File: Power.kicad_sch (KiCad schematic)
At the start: 26 parts, among them J401 KLDX-0202-B, J402 EBWA-02-B, Q401 MCU18P10Y-TP, U401 TPS7A2030PDBVR

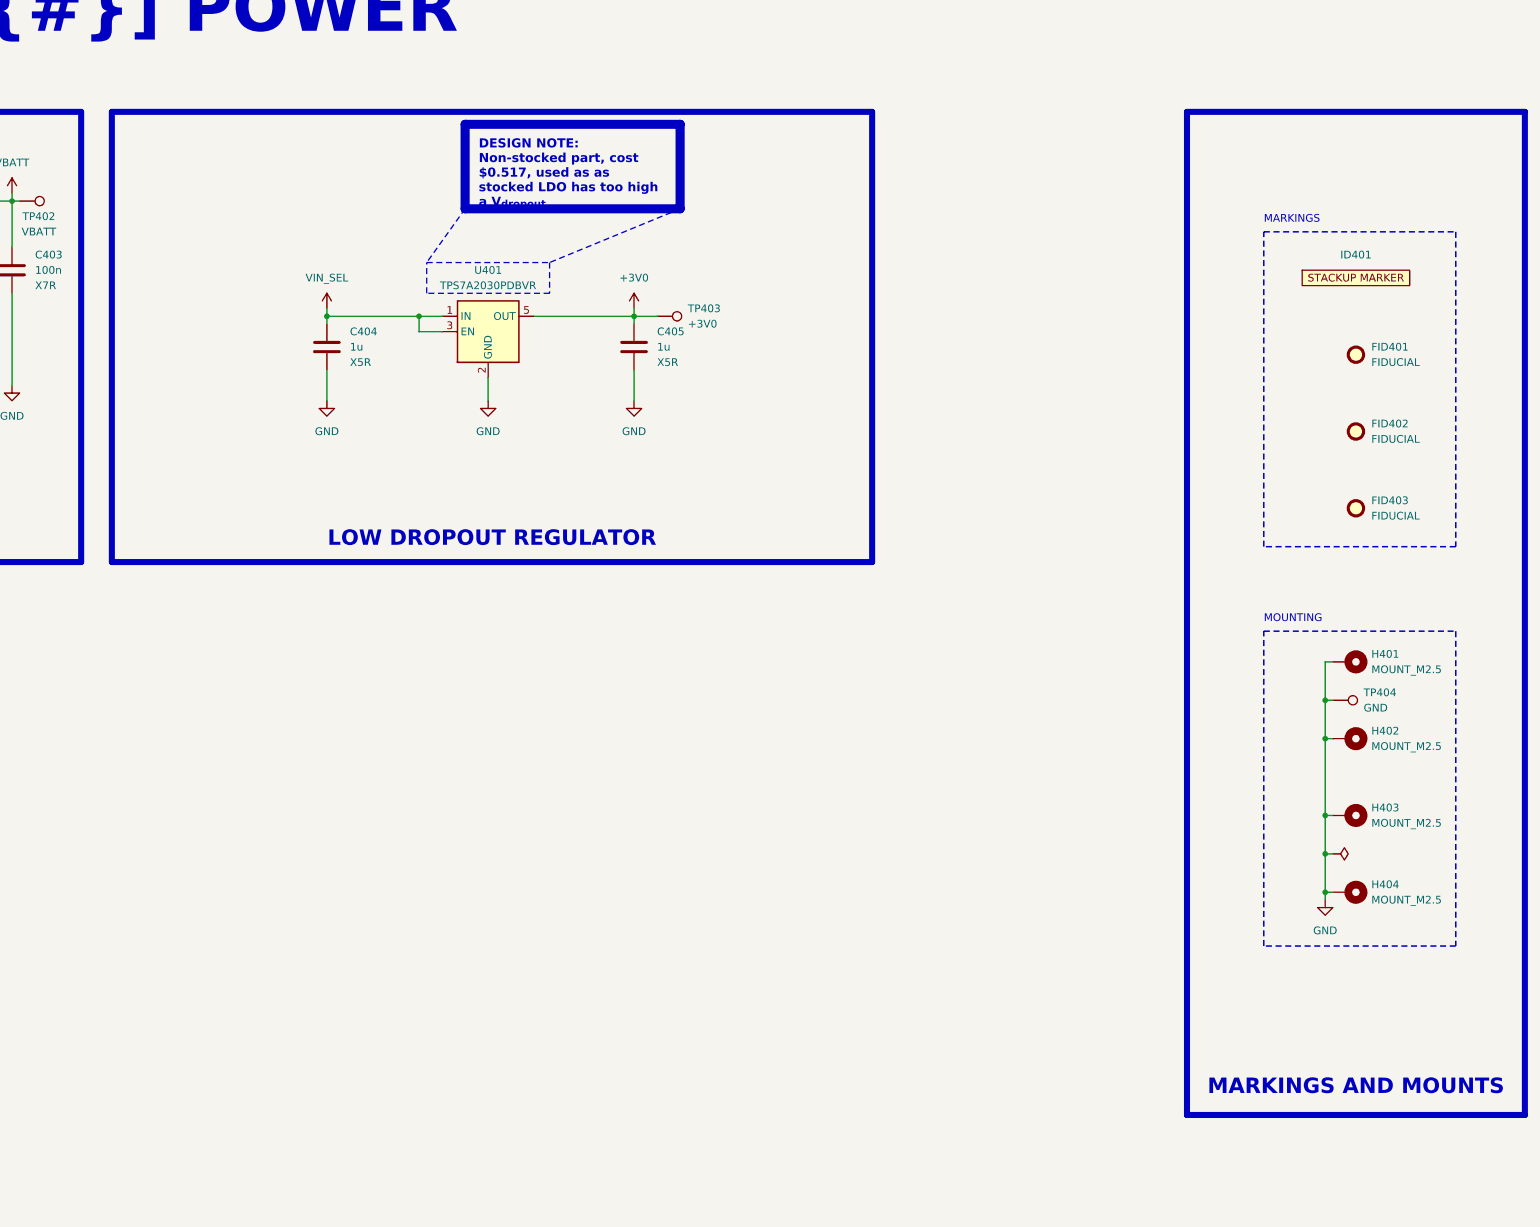
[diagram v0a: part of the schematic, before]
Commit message: feat: checked REV A
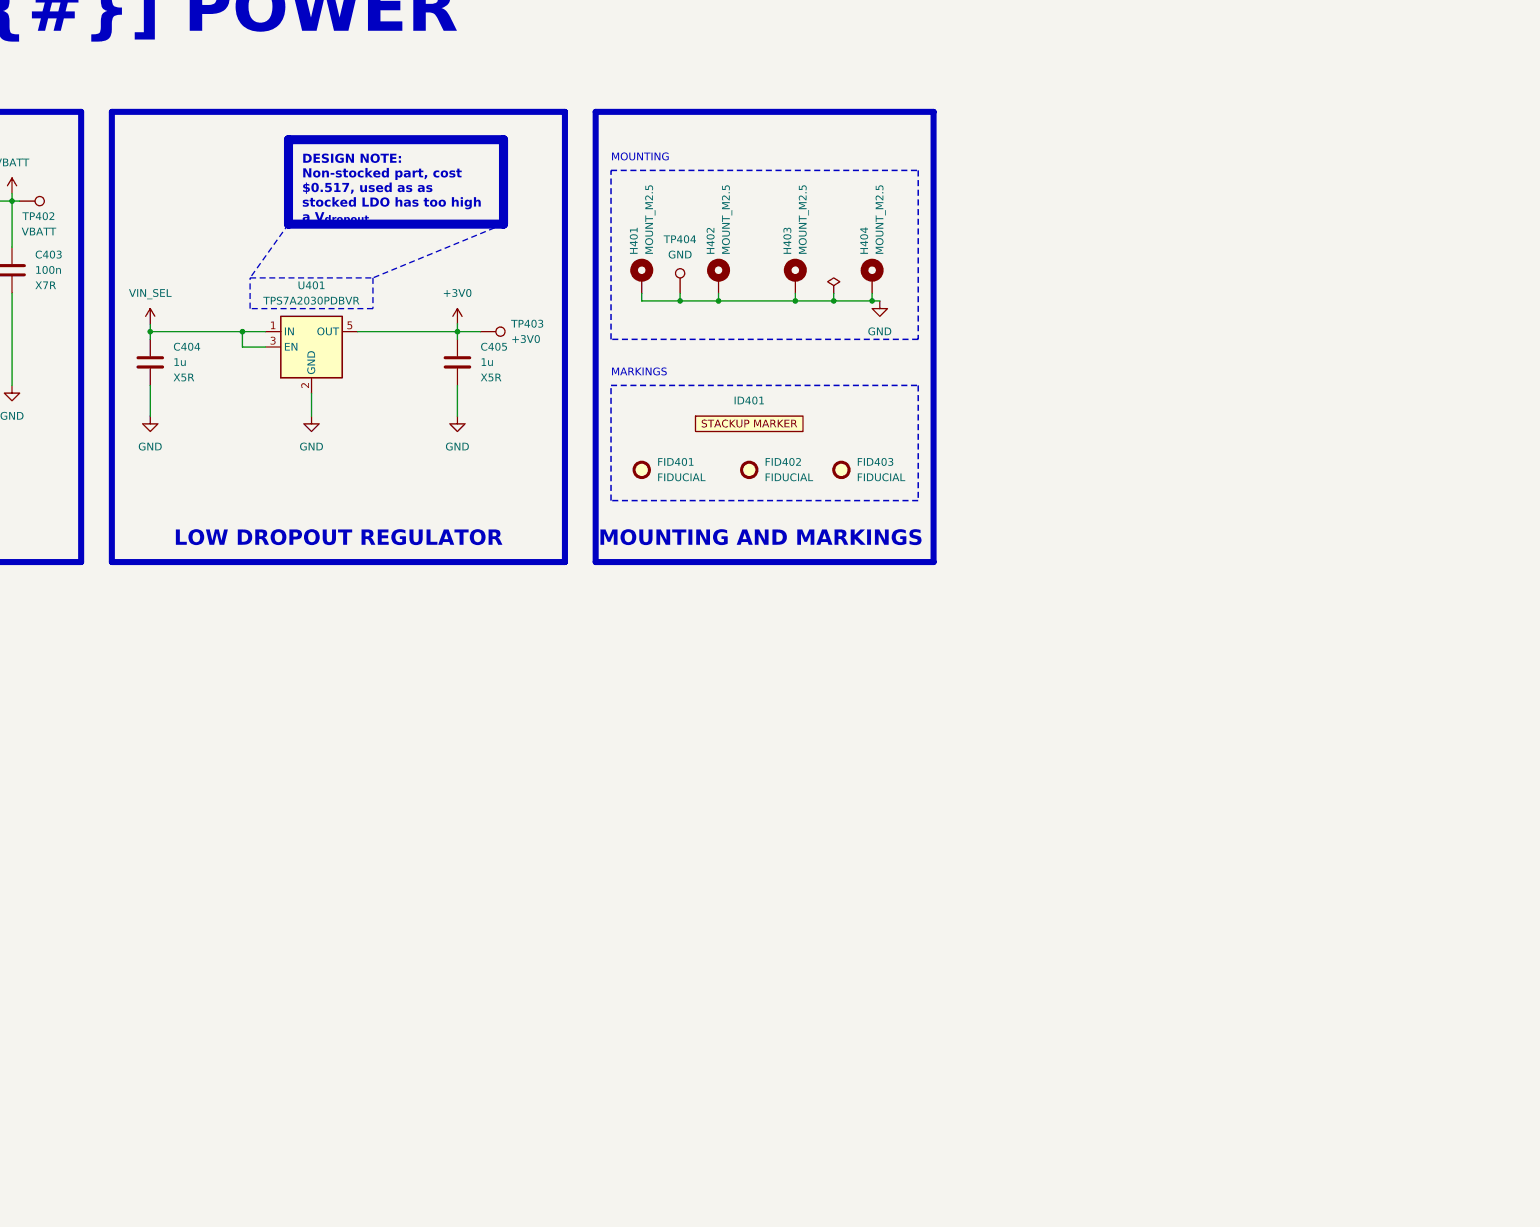
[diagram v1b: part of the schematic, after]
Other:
- moved on the sheet: C404, C405, FID401, FID402, FID403, H401, H402, H403, H404, ID401, TP403, TP404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
